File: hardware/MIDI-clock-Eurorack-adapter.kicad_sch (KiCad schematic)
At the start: 24 parts, among them J1 CLOCK, J2 RUN, J3 Conn_02x05_Odd_Even, Q1 2N3904, U1 TL072

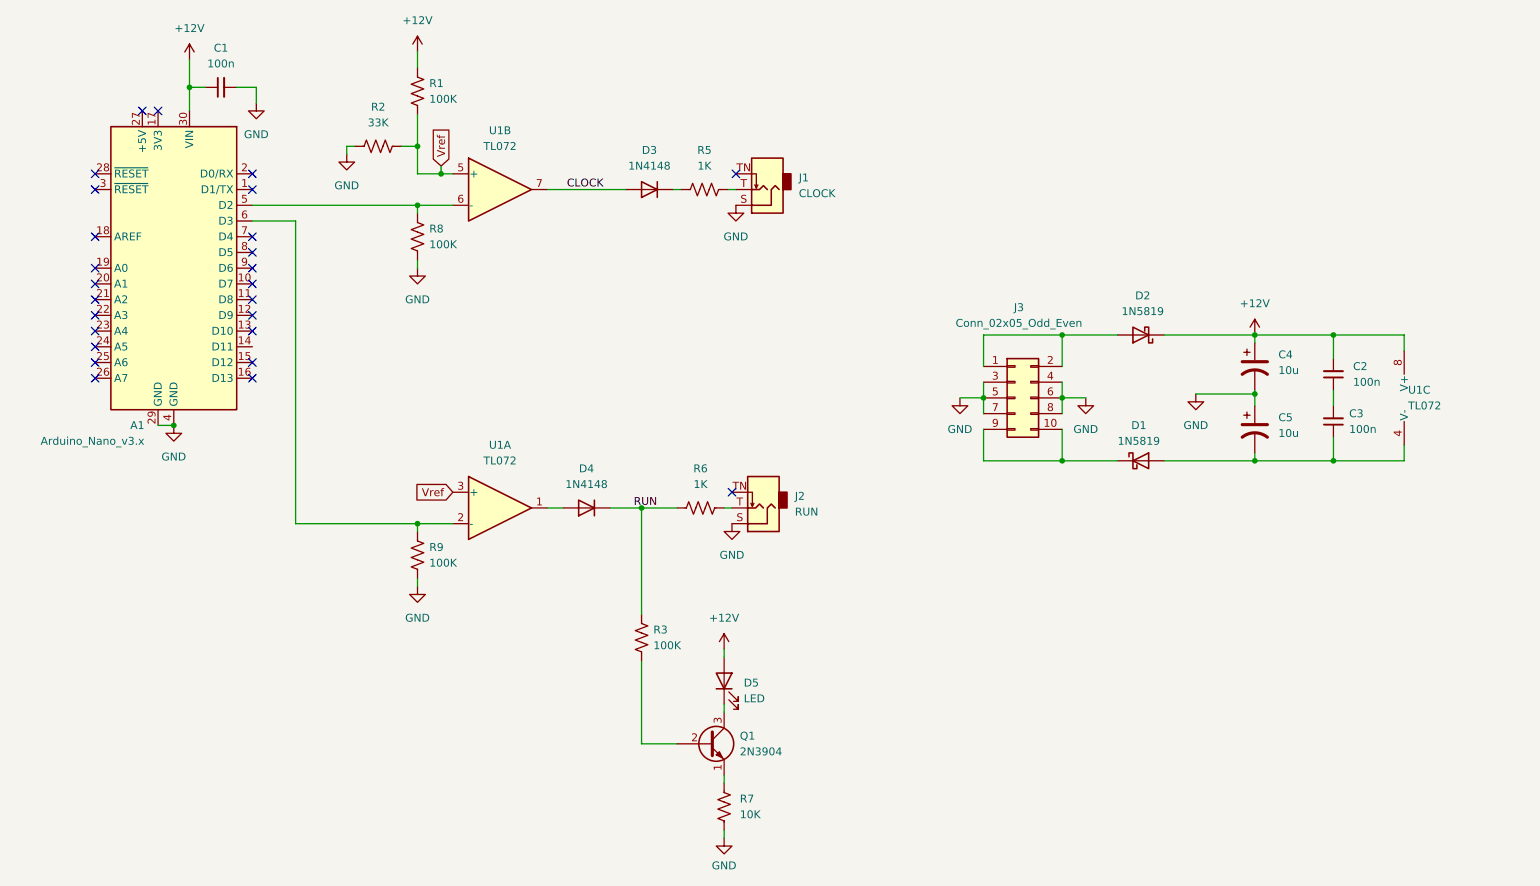
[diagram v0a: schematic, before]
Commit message: Update schematic
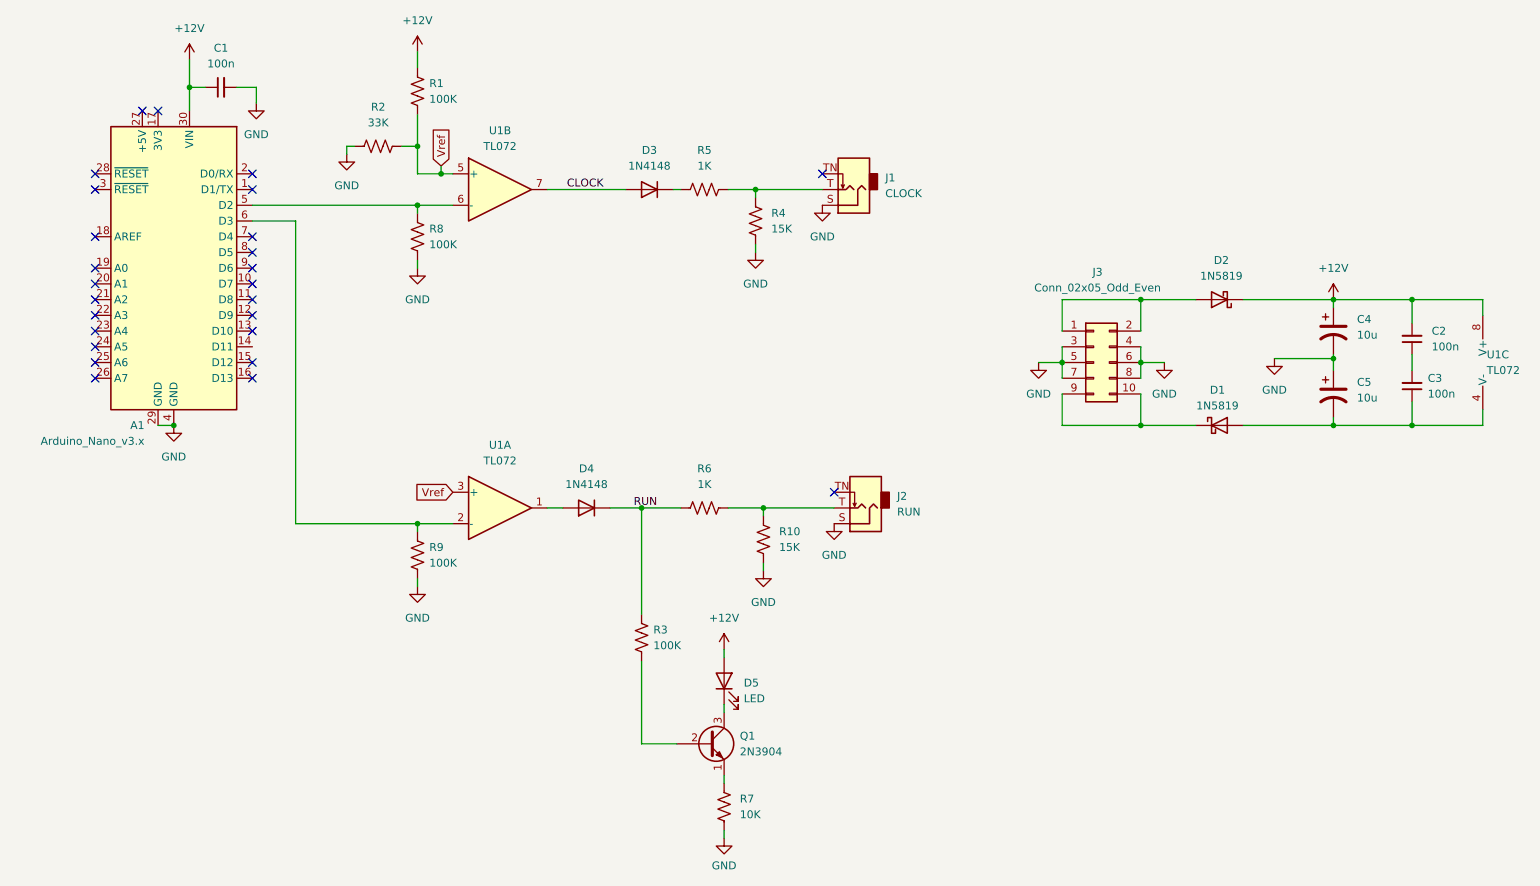
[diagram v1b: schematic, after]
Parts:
- added R10, R4: 15K, symbol Device:R_US
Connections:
- net GND: now also R10.1, R4.1
- net at J2.T, R6.2: now also R10.2
- net at J1.T, R5.2: now also R4.2
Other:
- moved on the sheet: C2, C3, C4, C5, D1, D2, J1, J2, J3, R6, U1C
